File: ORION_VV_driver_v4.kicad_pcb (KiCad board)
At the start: 4 copper layers, 52.4 x 123.1 mm, 158 parts, among them J1 Conn_01x01, J10 Conn_01x01, J11 Conn_01x02, J12 Conn_01x05, J13 Conn_01x05, J14 Conn_01x01, J15 Conn_01x02, J16 Conn_01x01, J17 Conn_01x01, J18 Conn_01x01, J19 Conn_01x01, J2 Conn_01x04, J20 Conn_01x01, J21 Conn_01x01, J22 Conn_01x01, J23 Conn_01x01, J3 Conn_01x04, J4 Conn_01x06, J5 Conn_01x07, J6 Conn_01x07, J7 Conn_01x01, J8 Conn_01x01, J9 Conn_01x01, Q1 IRF8721PBF-1, Q10 IRF8721PBF-1, Q11 IRF8721PBF-1, Q12 IRF8721PBF-1, Q2 IRF8721PBF-1, Q3 IRF8721PBF-1, Q4 IRF8721PBF-1, Q5 IRF8721PBF-1, Q6 IRF8721PBF-1, Q7 IRF8721PBF-1, Q8 IRF8721PBF-1, Q9 IRF8721PBF-1, SW1 SW_Push, SW2 SW_Push, SW3 SW_Push, SW4 SW_Push, SW5 SW_Push, U1 BD9G101G, U2 L78L33_SOT89, U3 MAX3051, U5 ZXCT108x, U6 ZXCT108x, Y1 Resonator

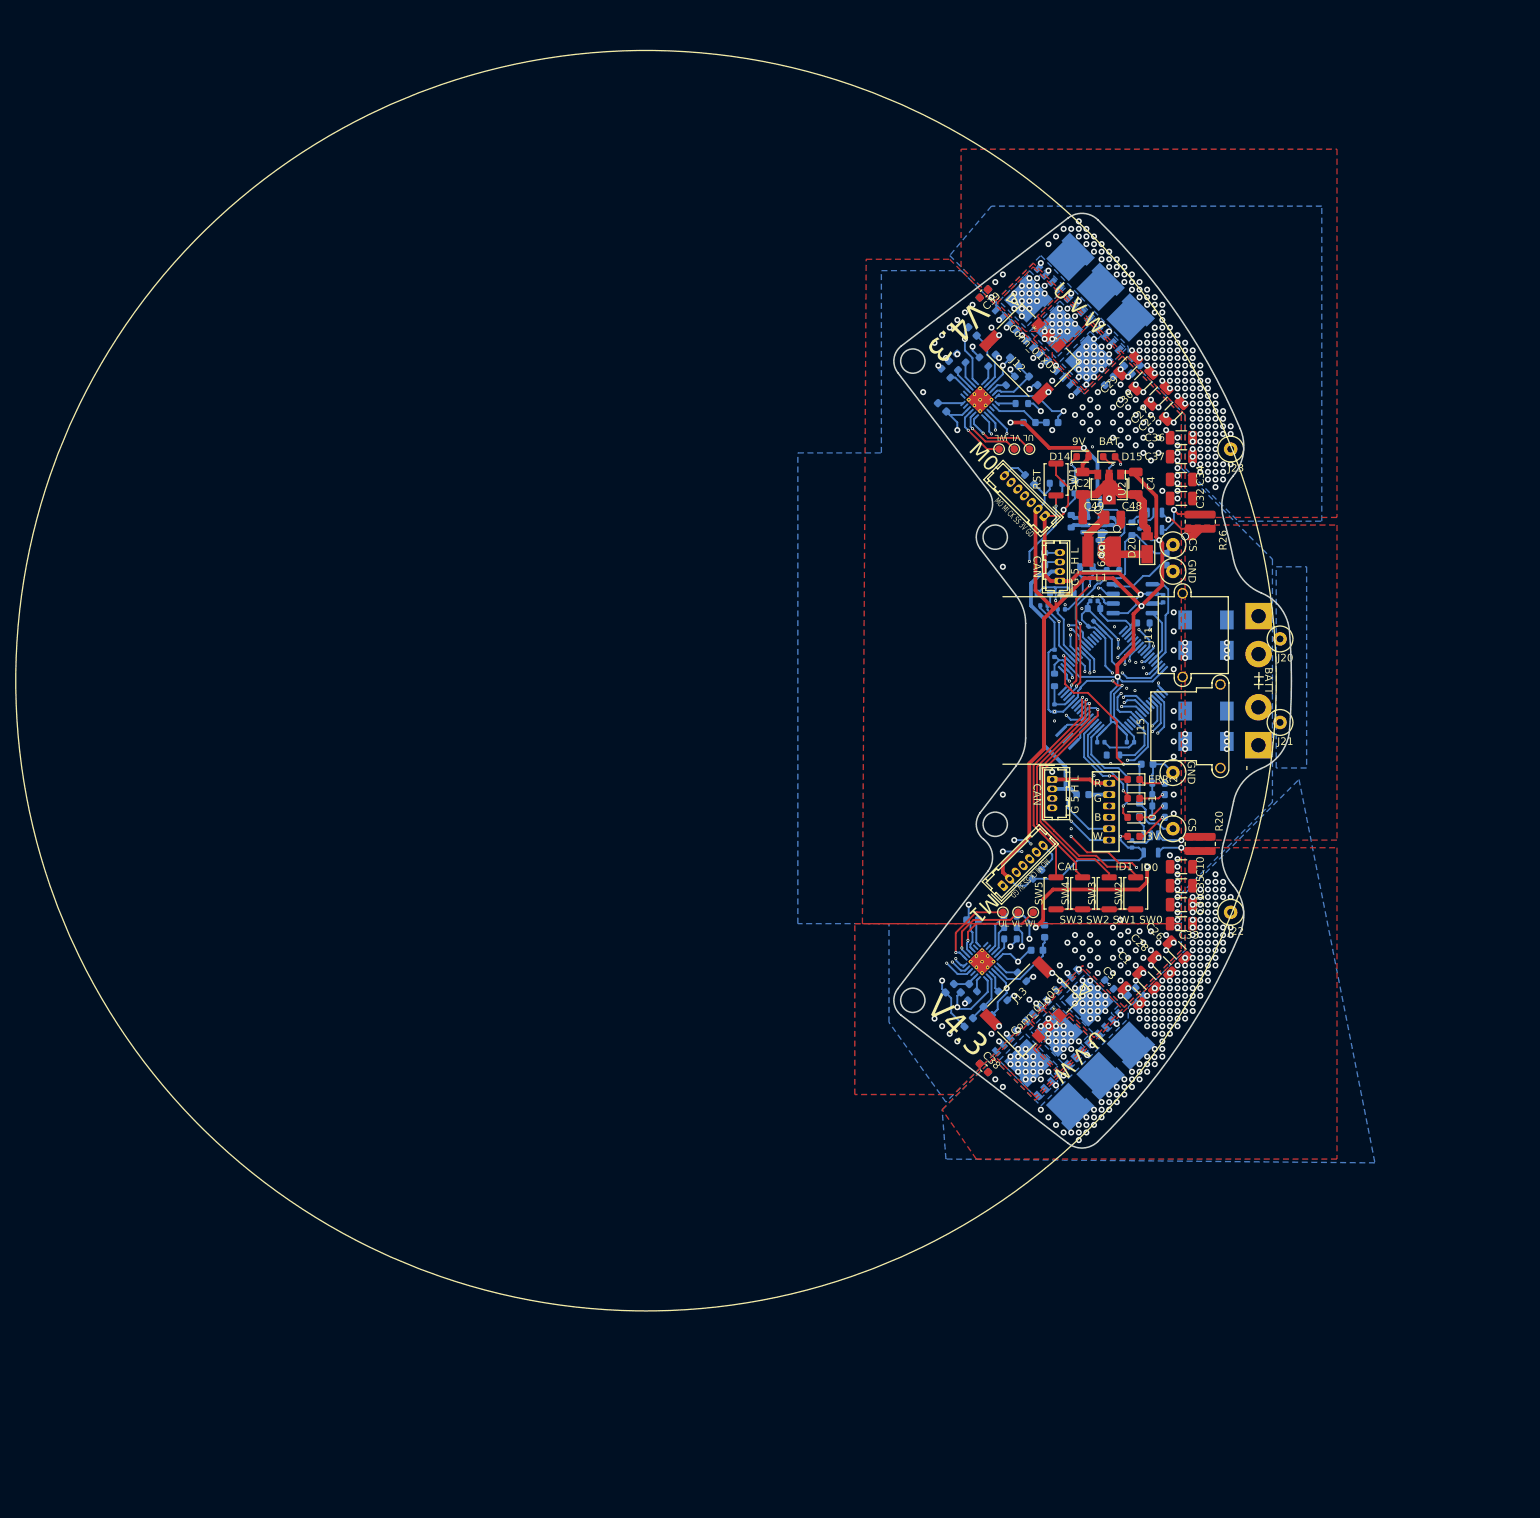
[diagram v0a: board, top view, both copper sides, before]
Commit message: 回転
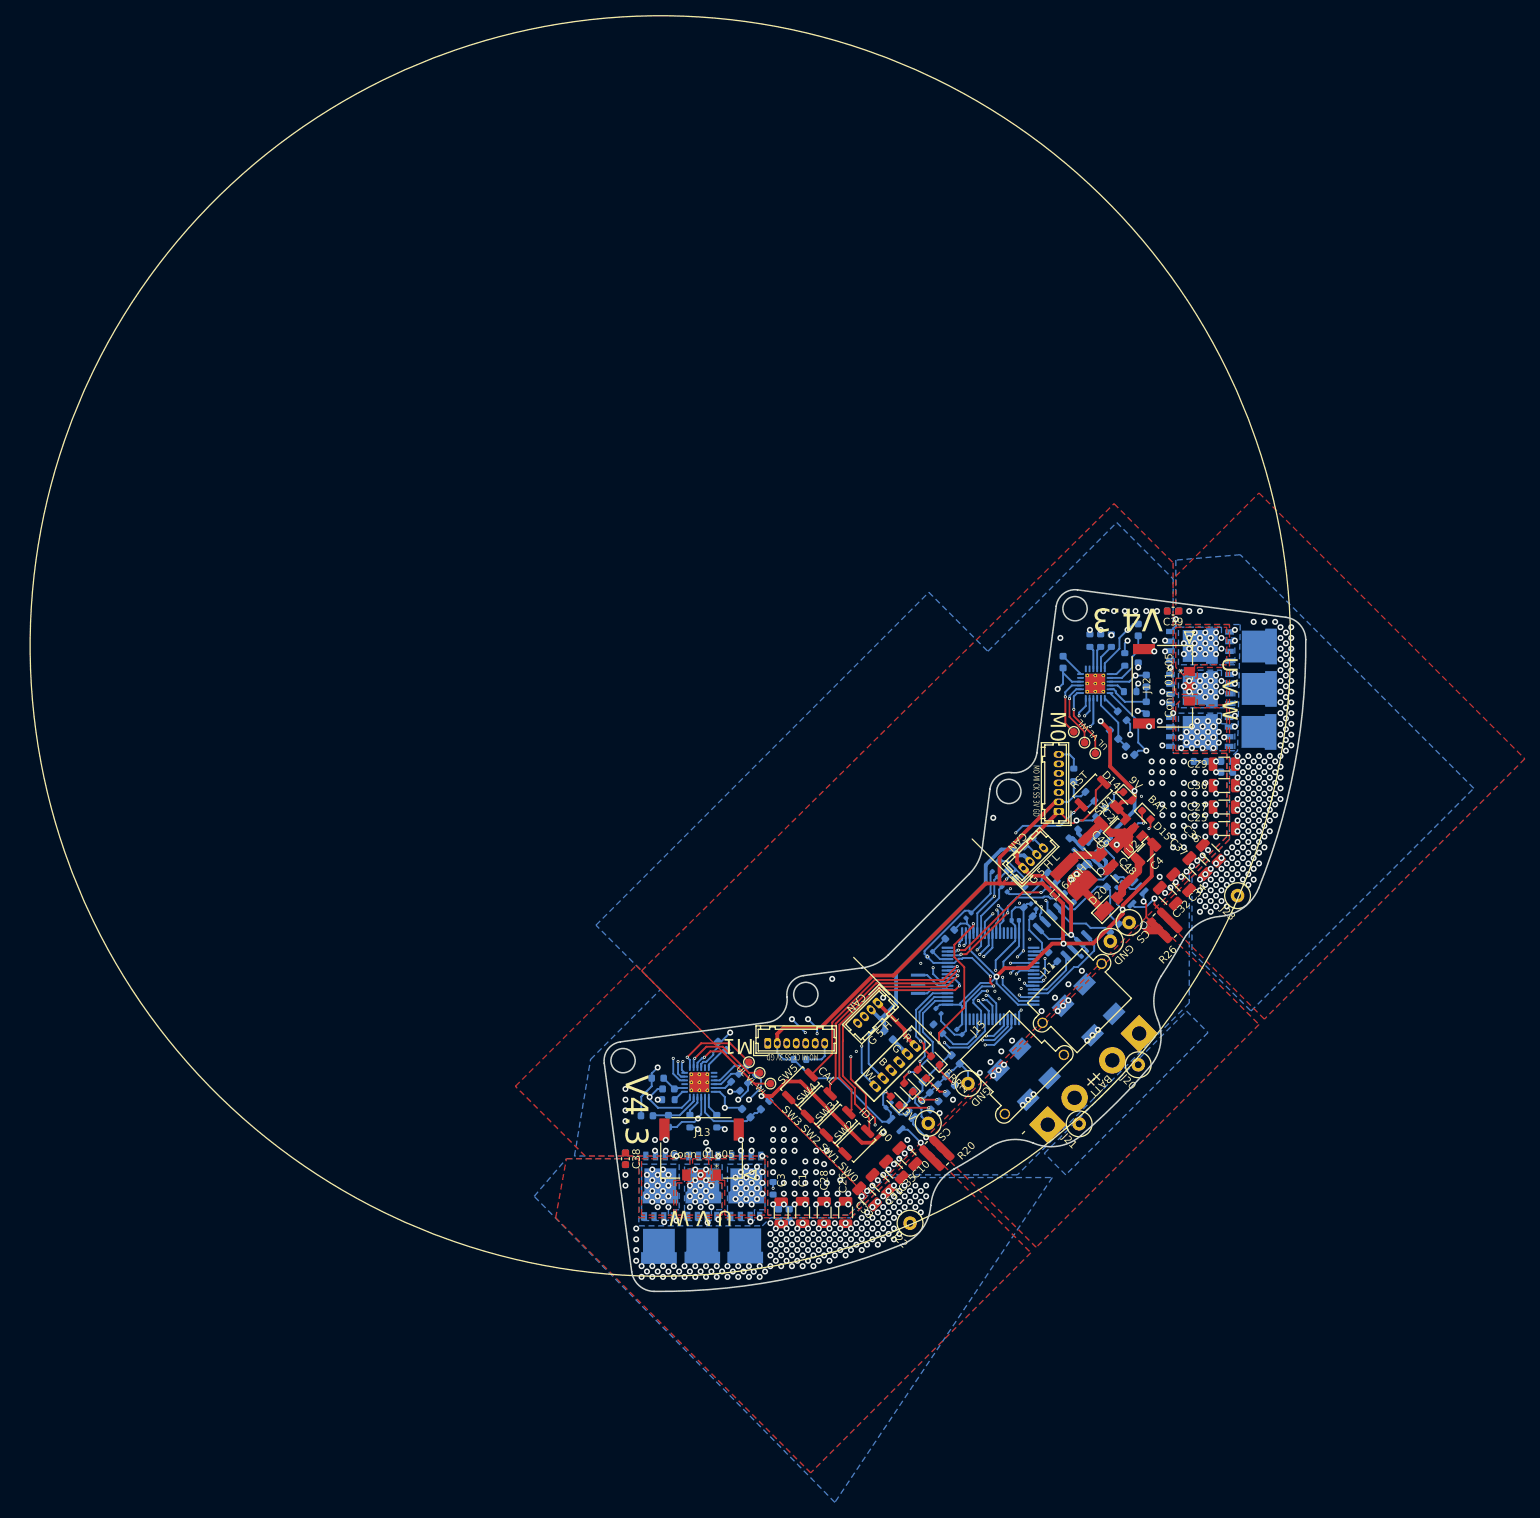
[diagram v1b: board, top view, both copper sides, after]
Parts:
- moved J21 59.1 mm to (111.0, 158.4), turned to -45 degrees
- moved J20 59.1 mm to (118.8, 150.6), turned to -45 degrees
- moved J23 58.8 mm to (131.9, 128.3), turned to -45 degrees
- moved J22 58.8 mm to (88.8, 171.4), turned to -45 degrees
- moved J11 57.2 mm to (118.9, 146.5), turned to 45 degrees
- moved J15 57.2 mm to (106.9, 158.5), turned to 45 degrees
- moved Q1 56.4 mm to (67.1, 173.3), turned to -90 degrees
- moved Q9 56.3 mm to (55.7, 173.4), turned to -90 degrees
- moved Q11 56.2 mm to (133.6, 106.7), turned to 0 degrees
- moved Q3 56.1 mm to (133.7, 95.5), turned to 0 degrees
- moved Q5 56.1 mm to (61.4, 173.3), turned to -90 degrees
- moved Q7 56.0 mm to (133.7, 101.1), turned to 0 degrees
- moved C26 55.7 mm to (80.3, 170.0), turned to 90 degrees
- moved C25 55.4 mm to (130.1, 119.5), turned to 180 degrees
- moved C28 55.2 mm to (77.5, 170.0), turned to 90 degrees
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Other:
- board size 52.4 x 123.1 mm -> 92.4 x 92.4 mm
